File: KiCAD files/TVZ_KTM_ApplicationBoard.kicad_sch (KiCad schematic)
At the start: 52 parts, among them J1 Conn_02x19_Odd_Even, J2 Conn_02x19_Odd_Even, J3 Conn_02x19_Odd_Even, J4 Conn_02x19_Odd_Even, SW1 OS102011MS2QN1, SW2 OS102011MS2QN1, SW3 OS102011MS2QN1, SW4 OS102011MS2QN1, U1 LM75B, U2 MCP2551-I-P, U3 MCP2551-I-P

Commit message: update
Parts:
- D1, D10, D11, D12, D2, D3, D4, D5, D6, D7, D8, D9: footprint LED_THT:LED_D5.0mm -> LED_SMD:LED_1206_3216Metric
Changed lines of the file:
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@@
       (effects (font (size 1.27 1.27)) (justify right))
     )
-    (property "Footprint" "LED_THT:LED_D5.0mm" (id 2) (at 68.58 87.63 90)
+    (property "Footprint" "LED_SMD:LED_1206_3216Metric" (id 2) (at 68.58 87.63 90)
       (effects (font (size 1.27 1.27)) hide)
     )
@@
       (effects (font (size 1.27 1.27)) (justify right))
     )
-    (property "Footprint" "LED_THT:LED_D5.0mm" (id 2) (at 60.96 87.63 90)
+    (property "Footprint" "LED_SMD:LED_1206_3216Metric" (id 2) (at 60.96 87.63 90)
       (effects (font (size 1.27 1.27)) hide)
     )
@@
       (effects (font (size 1.27 1.27)) (justify right))
     )
-    (property "Footprint" "LED_THT:LED_D5.0mm" (id 2) (at 88.265 86.995 90)
+    (property "Footprint" "LED_SMD:LED_1206_3216Metric" (id 2) (at 88.265 86.995 90)
       (effects (font (size 1.27 1.27)) hide)
     )
@@
       (effects (font (size 1.27 1.27)) (justify right))
     )
-    (property "Footprint" "LED_THT:LED_D5.0mm" (id 2) (at 14.605 87.63 90)
+    (property "Footprint" "LED_SMD:LED_1206_3216Metric" (id 2) (at 14.605 87.63 90)
       (effects (font (size 1.27 1.27)) hide)
     )
@@
       (effects (font (size 1.27 1.27)) (justify right))
     )
-    (property "Footprint" "LED_THT:LED_D5.0mm" (id 2) (at 76.2 87.63 90)
+    (property "Footprint" "LED_SMD:LED_1206_3216Metric" (id 2) (at 76.2 87.63 90)
       (effects (font (size 1.27 1.27)) hide)
     )
@@
       (effects (font (size 1.27 1.27)) (justify right))
     )
-    (property "Footprint" "LED_THT:LED_D5.0mm" (id 2) (at 95.25 86.995 90)
+    (property "Footprint" "LED_SMD:LED_1206_3216Metric" (id 2) (at 95.25 86.995 90)
       (effects (font (size 1.27 1.27)) hide)
     )
@@
       (effects (font (size 1.27 1.27)) (justify right))
     )
-    (property "Footprint" "LED_THT:LED_D5.0mm" (id 2) (at 53.975 87.63 90)
+    (property "Footprint" "LED_SMD:LED_1206_3216Metric" (id 2) (at 53.975 87.63 90)
       (effects (font (size 1.27 1.27)) hide)
     )
@@
       (effects (font (size 1.27 1.27)) (justify right))
     )
-    (property "Footprint" "LED_THT:LED_D5.0mm" (id 2) (at 102.87 86.995 90)
+    (property "Footprint" "LED_SMD:LED_1206_3216Metric" (id 2) (at 102.87 86.995 90)
       (effects (font (size 1.27 1.27)) hide)
     )
@@
       (effects (font (size 1.27 1.27)) (justify right))
     )
-    (property "Footprint" "LED_THT:LED_D5.0mm" (id 2) (at 33.655 87.63 90)
+    (property "Footprint" "LED_SMD:LED_1206_3216Metric" (id 2) (at 33.655 87.63 90)
       (effects (font (size 1.27 1.27)) hide)
     )
@@
       (effects (font (size 1.27 1.27)) (justify right))
     )
-    (property "Footprint" "LED_THT:LED_D5.0mm" (id 2) (at 24.13 87.63 90)
+    (property "Footprint" "LED_SMD:LED_1206_3216Metric" (id 2) (at 24.13 87.63 90)
       (effects (font (size 1.27 1.27)) hide)
     )
@@
       (effects (font (size 1.27 1.27)) (justify right))
     )
-    (property "Footprint" "LED_THT:LED_D5.0mm" (id 2) (at 43.18 87.63 90)
+    (property "Footprint" "LED_SMD:LED_1206_3216Metric" (id 2) (at 43.18 87.63 90)
       (effects (font (size 1.27 1.27)) hide)
     )
@@
       (effects (font (size 1.27 1.27)) (justify right))
     )
-    (property "Footprint" "LED_THT:LED_D5.0mm" (id 2) (at 110.49 86.995 90)
+    (property "Footprint" "LED_SMD:LED_1206_3216Metric" (id 2) (at 110.49 86.995 90)
       (effects (font (size 1.27 1.27)) hide)
     )
@@
     )
     (path "/3d19cfb4-61fb-4342-b2d6-f42e693be3a5"
-      (reference "D1") (unit 1) (value "BLUE") (footprint "LED_THT:LED_D5.0mm")
+      (reference "D1") (unit 1) (value "BLUE") (footprint "LED_SMD:LED_1206_3216Metric")
     )
     (path "/7afe3747-525c-42e5-93d7-fe72e6eb0f5a"
-      (reference "D2") (unit 1) (value "BLUE") (footprint "LED_THT:LED_D5.0mm")
+      (reference "D2") (unit 1) (value "BLUE") (footprint "LED_SMD:LED_1206_3216Metric")
     )
     (path "/ce01e21d-824d-43d0-b5c6-aed8b80d67e6"
-      (reference "D3") (unit 1) (value "BLUE") (footprint "LED_THT:LED_D5.0mm")
+      (reference "D3") (unit 1) (value "BLUE") (footprint "LED_SMD:LED_1206_3216Metric")
     )
     (path "/fa7611f7-c799-43f9-b83c-caa62f2095bf"
-      (reference "D4") (unit 1) (value "BLUE") (footprint "LED_THT:LED_D5.0mm")
+      (reference "D4") (unit 1) (value "BLUE") (footprint "LED_SMD:LED_1206_3216Metric")
     )
     (path "/3f714e49-2c98-4c5c-9a0e-1b7ac4aa1ac9"
-      (reference "D5") (unit 1) (value "GREEN") (footprint "LED_THT:LED_D5.0mm")
+      (reference "D5") (unit 1) (value "GREEN") (footprint "LED_SMD:LED_1206_3216Metric")
     )
     (path "/df35f80b-ec52-4a20-8bfd-16dbb009585b"
-      (reference "D6") (unit 1) (value "GREEN") (footprint "LED_THT:LED_D5.0mm")
+      (reference "D6") (unit 1) (value "GREEN") (footprint "LED_SMD:LED_1206_3216Metric")
     )
     (path "/db6cb11f-e683-48e5-bbbc-aa35d75403d5"
-      (reference "D7") (unit 1) (value "GREEN") (footprint "LED_THT:LED_D5.0mm")
+      (reference "D7") (unit 1) (value "GREEN") (footprint "LED_SMD:LED_1206_3216Metric")
     )
     (path "/e97b4c0d-ef6a-4ceb-b1e1-5c85e7f6a874"
-      (reference "D8") (unit 1) (value "GREEN") (footprint "LED_THT:LED_D5.0mm")
+      (reference "D8") (unit 1) (value "GREEN") (footprint "LED_SMD:LED_1206_3216Metric")
     )
     (path "/b8bd83b0-d5a1-4d6e-a11d-92517f315197"
-      (reference "D9") (unit 1) (value "RED") (footprint "LED_THT:LED_D5.0mm")
+      (reference "D9") (unit 1) (value "RED") (footprint "LED_SMD:LED_1206_3216Metric")
     )
     (path "/3b749e35-8de6-4a7f-8659-ea682cc9233a"
-      (reference "D10") (unit 1) (value "RED") (footprint "LED_THT:LED_D5.0mm")
+      (reference "D10") (unit 1) (value "RED") (footprint "LED_SMD:LED_1206_3216Metric")
     )
     (path "/0dc03840-c27f-46dc-948b-4b6ed1aa0b11"
-      (reference "D11") (unit 1) (value "RED") (footprint "LED_THT:LED_D5.0mm")
+      (reference "D11") (unit 1) (value "RED") (footprint "LED_SMD:LED_1206_3216Metric")
     )
     (path "/4593df50-01a0-49b2-b14f-f46663c1a9aa"
-      (reference "D12") (unit 1) (value "RED") (footprint "LED_THT:LED_D5.0mm")
+      (reference "D12") (unit 1) (value "RED") (footprint "LED_SMD:LED_1206_3216Metric")
     )
     (path "/2f3ec83e-bbf5-4e22-aae3-b46a96e60126"

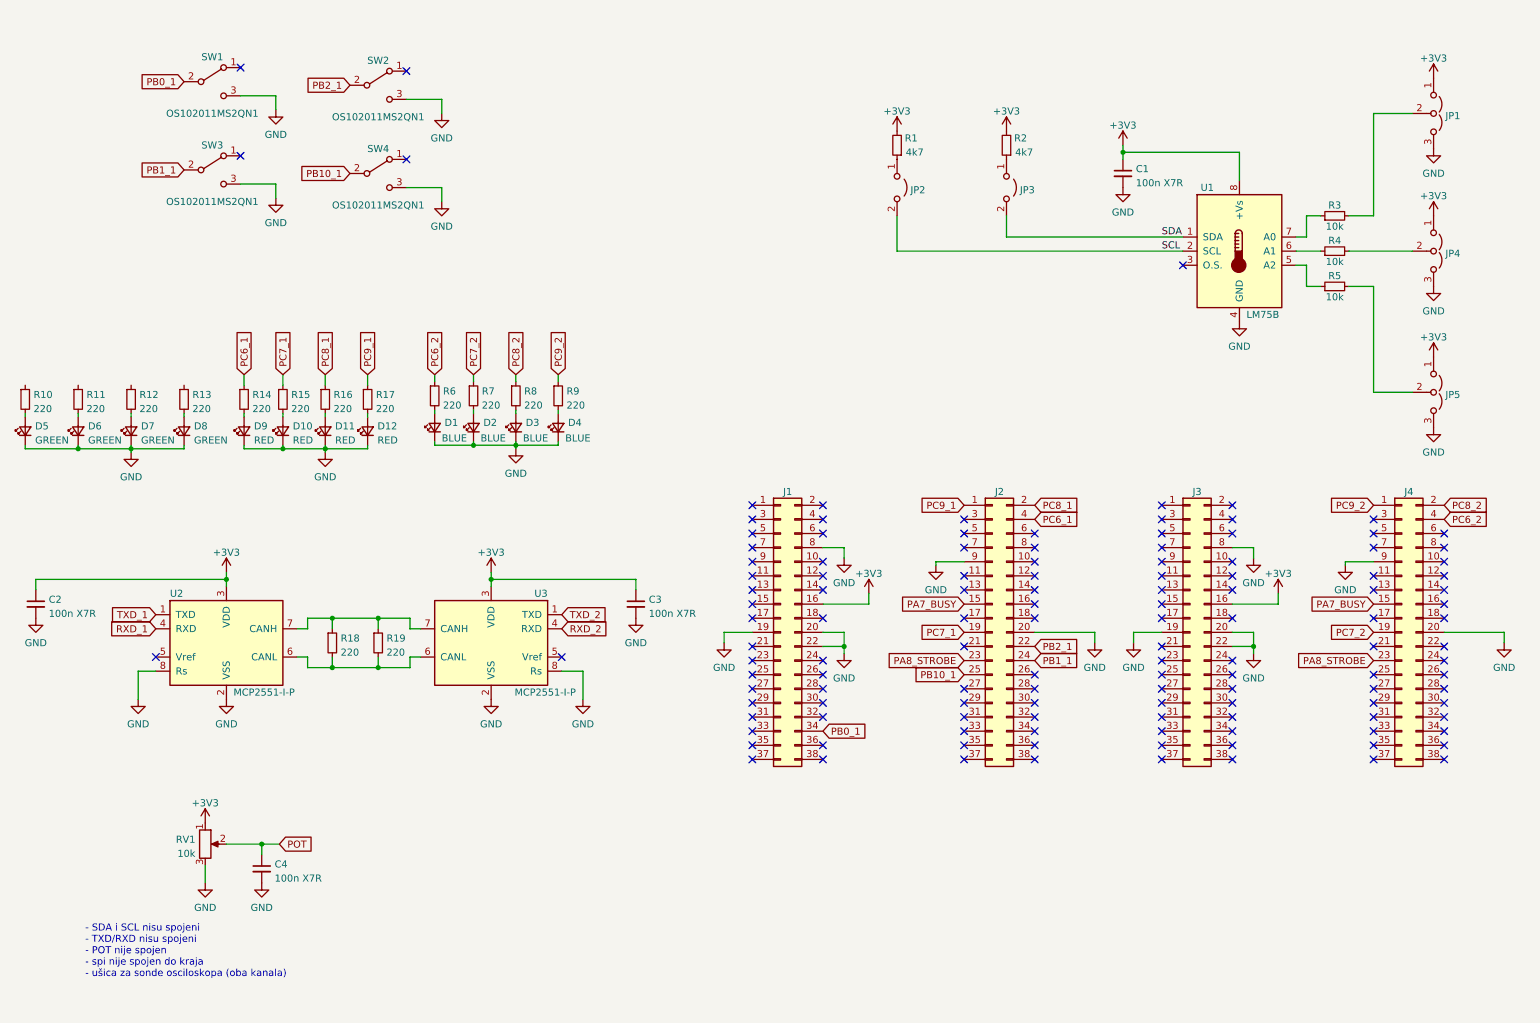
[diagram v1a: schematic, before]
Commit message: update
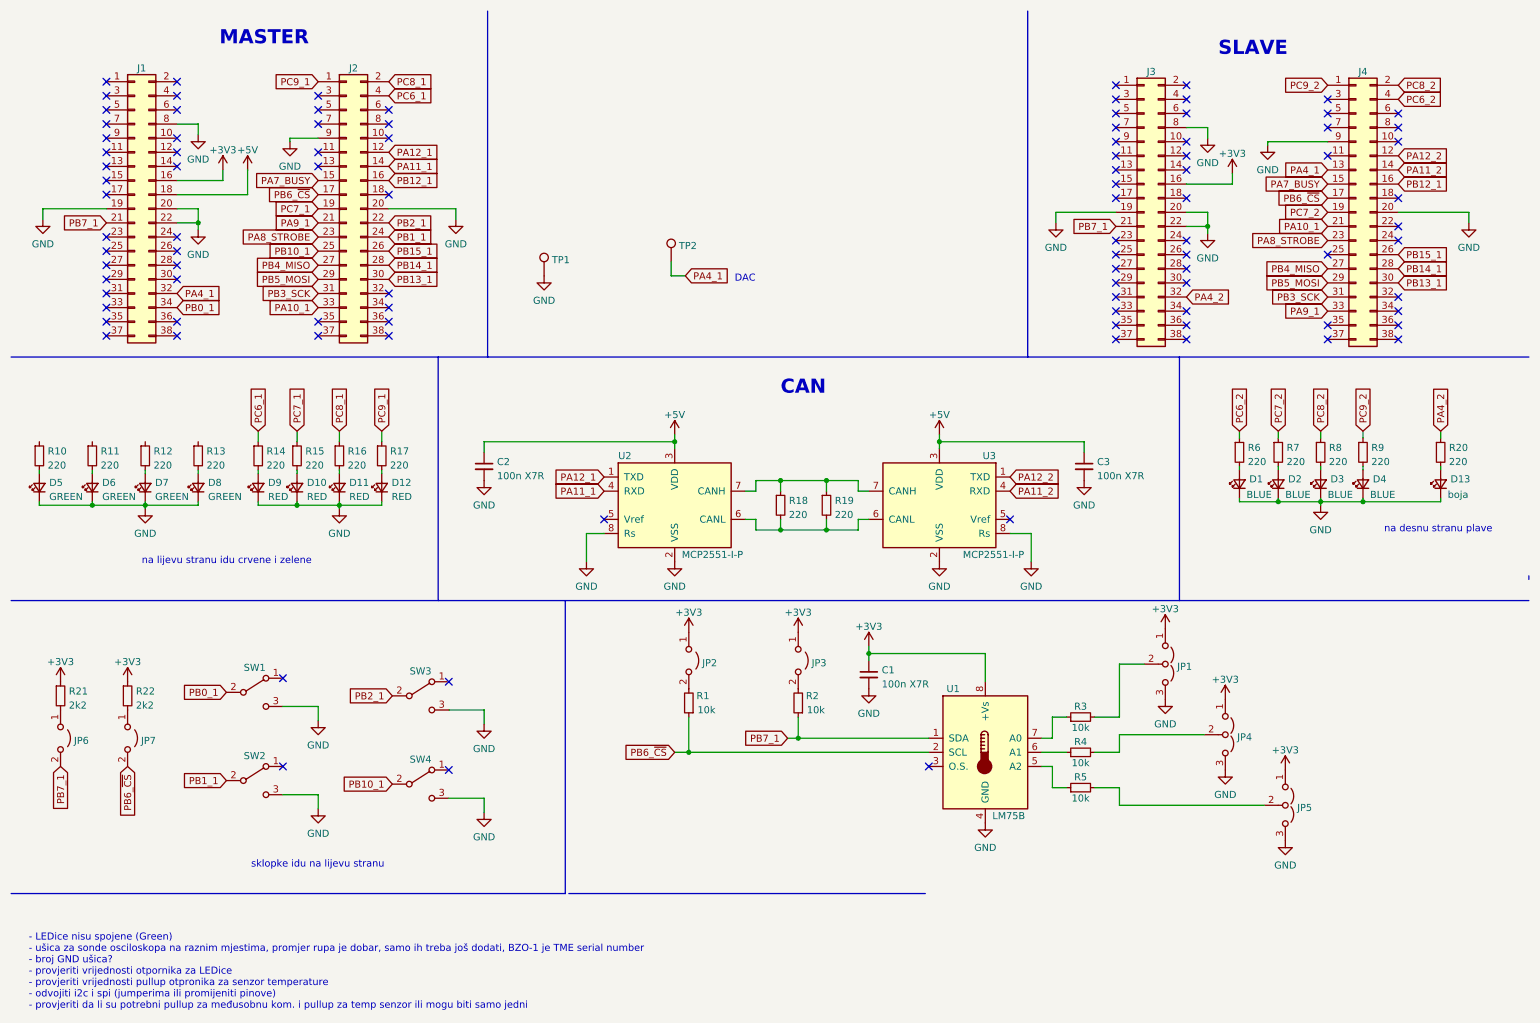
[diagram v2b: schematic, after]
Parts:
- removed C4: 100n X7R, Capacitor_SMD:C_0603_1608Metric, symbol Device:C_Small
- removed RV1: 10k, Footprints:Potentiometer_Bourns_3386P_Vertical, symbol Device:R_Potentiometer
- added D13: boja, LED_SMD:LED_1206_3216Metric, symbol Device:LED_Small
- added JP6, JP7: Jumper_2_Open, Connector_PinHeader_2.54mm:PinHeader_1x02_P2.54mm_Vertical, symbol Jumper:Jumper_2_Open
- added R20: 220, Resistor_SMD:R_0805_2012Metric, symbol Device:R_Small
- added R21, R22: 2k2, Resistor_SMD:R_0805_2012Metric, symbol Device:R_Small
- added TP1, TP2: TestPoint, TestPoint:TestPoint_THTPad_D3.0mm_Drill1.5mm, symbol Connector:TestPoint
- C1, C2, C3: footprint Capacitor_SMD:C_0603_1608Metric -> Capacitor_SMD:C_0805_2012Metric
- R1, R2: value 4k7 -> 10k; footprint Resistor_SMD:R_0603_1608Metric -> Resistor_SMD:R_0805_2012Metric
- R10, R11, R12, R13, R14, R15, R16, R17, R18, R19, R3, R4, R5, R6, R7, R8, R9: footprint Resistor_SMD:R_0603_1608Metric -> Resistor_SMD:R_0805_2012Metric
- SW1, SW4: value OS102011MS2QN1 -> EG1271A; footprint Footprints:OS102011MS2QN1 -> Footprint:EG1271A
- SW2: renamed from SW3; value OS102011MS2QN1 -> EG1271A; footprint Footprints:OS102011MS2QN1 -> Footprint:EG1271A
- SW3: renamed from SW2; value OS102011MS2QN1 -> EG1271A; footprint Footprints:OS102011MS2QN1 -> Footprint:EG1271A
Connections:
- net RXD_1 is gone; now on net PA11_1: U2.4 (RXD)
- net RXD_2 is gone; now on net PA11_2: U3.4 (RXD)
- net TXD_1 is gone; now on net PA12_1: U2.1 (TXD)
- net TXD_2 is gone; now on net PA12_2: U3.1 (TXD)
- net +3V3: now also JP2.1 (A), JP3.1 (A), R21.1, R22.1; no longer C2.1, C3.1, R1.2, R2.2, U2.3 (VDD), U3.3 (VDD)
- net GND: now also D13.1 (K), TP1.1
- net PB7_1: now reaches J3.21 (Pin_21)
- net PB7_1: now also J1.21 (Pin_21), R2.1, U1.1 (SDA), JP6.2 (B)
- net PA4_2: now reaches J3.32 (Pin_32)
- net PA4_2: now also R20.1
- net PA12_2: now reaches J4.12 (Pin_12)
- net PA4_1: now reaches J4.13 (Pin_13)
- net PA4_1: now also J1.32 (Pin_32), TP2.1
- net PA11_2: now reaches J4.14 (Pin_14)
- net PB12_1: now reaches J4.16 (Pin_16)
- net PB12_1: now also J2.16 (Pin_16)
- net PB6_~{CS}: now reaches J4.17 (Pin_17)
- net PB6_~{CS}: now also J2.17 (Pin_17), R1.1, U1.2 (SCL), JP7.2 (B)
- net PA10_1: now reaches J4.21 (Pin_21)
- net PA10_1: now also J2.33 (Pin_33)
- net PB15_1: now reaches J4.26 (Pin_26)
- net PB15_1: now also J2.26 (Pin_26)
- net PB4_MISO: now reaches J4.27 (Pin_27)
- net PB4_MISO: now also J2.27 (Pin_27)
- net PB14_1: now reaches J4.28 (Pin_28)
- net PB14_1: now also J2.28 (Pin_28)
- net PB5_MOSI: now reaches J4.29 (Pin_29)
- net PB5_MOSI: now also J2.29 (Pin_29)
- net PB13_1: now reaches J4.30 (Pin_30)
- net PB13_1: now also J2.30 (Pin_30)
- net PB3_SCK: now reaches J4.31 (Pin_31)
- net PB3_SCK: now also J2.31 (Pin_31)
- net PA9_1: now reaches J4.33 (Pin_33)
- net PA9_1: now also J2.21 (Pin_21)
- net +5V: now reaches J1.18 (Pin_18)
- net +5V: now also C2.1, C3.1, U2.3 (VDD), U3.3 (VDD)
- net PA12_1: now reaches J2.12 (Pin_12)
- net PA11_1: now reaches J2.14 (Pin_14)
- net SCL: no longer names the net of JP2.2 (B)
- net SCL: now also R1.2; no longer U1.2 (SCL)
- net SDA: no longer names the net of JP3.2 (B)
- net SDA: now also R2.2; no longer U1.1 (SDA)
- new net: JP6.1 (A), R21.2
- new net: D13.2 (A), R20.2
- new net: JP7.1 (A), R22.2
- no-connect marks 129 -> 99
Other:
- note added: "- LEDice nisu spojene (Green) - ušica za sonde osciloskopa na raznim mjestima, promjer rupa je dobar, samo ih treba još dodati, BZO-1 je TME serial number - broj GND ušica? - provjeriti vrijednosti otpornika za LEDice - provjeriti vrijednosti pullup otpronika za senzor temperature - odvojiti i2c i spi (jumperima ili promijeniti pinove) - provjeriti da li su potrebni pullup za međusobnu kom. i pul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"
- note added: "CAN"
- note added: "DAC"
- note added: "MASTER"
- note added: "SLAVE"
- note added: "na desnu stranu plave"
- note added: "na lijevu stranu idu crvene i zelene"
- note added: "sklopke idu na lijevu stranu"
- note removed: "- SDA i SCL nisu spojeni - TXD/RXD nisu spojeni - POT nije spojen - spi nije spojen do kraja - ušica za sonde osciloskopa (oba kanala)"
- moved on the sheet: C1, C2, C3, D1, D10, D11, D12, D2, D3, D4, D5, D6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
